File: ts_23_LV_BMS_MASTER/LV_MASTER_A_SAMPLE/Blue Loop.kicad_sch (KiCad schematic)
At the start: 16 parts, among them Q1 STD7NK40Z, Q2 STD7NK40Z, U9 ADUM3221

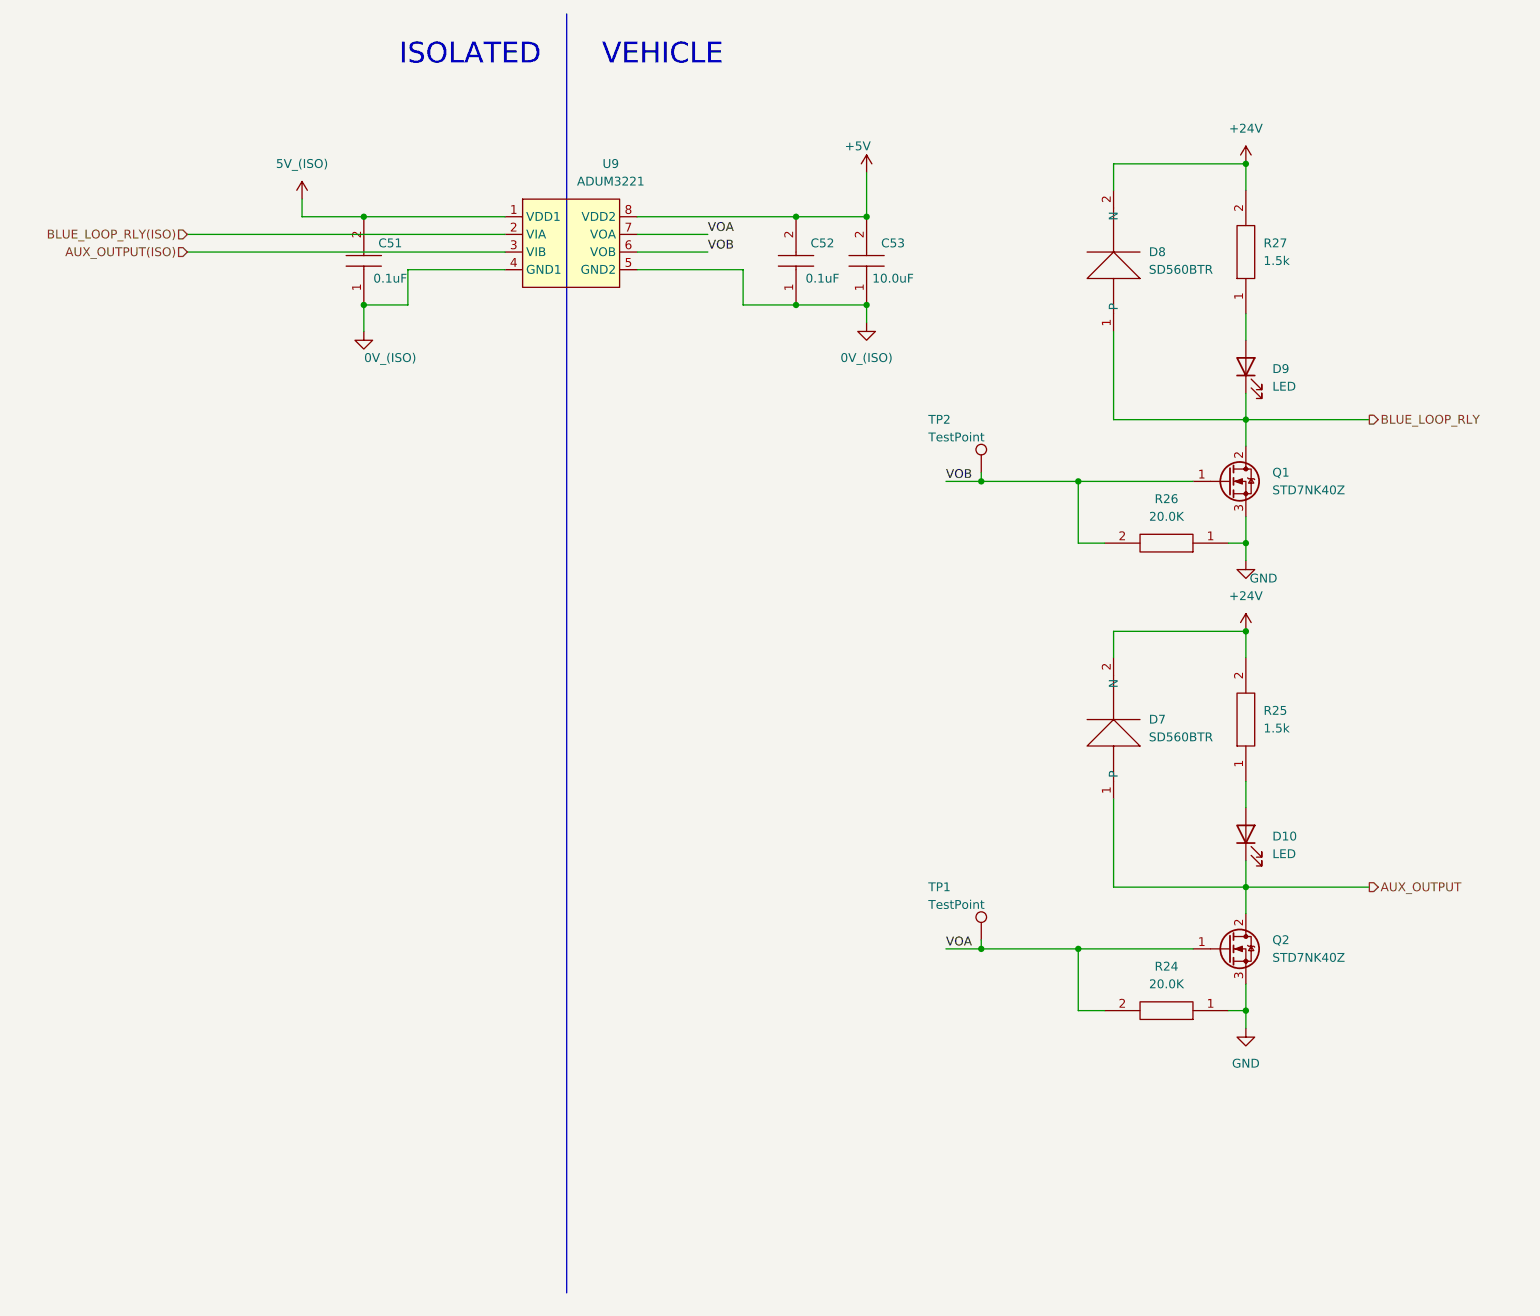
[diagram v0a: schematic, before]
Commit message: Final Changes to board
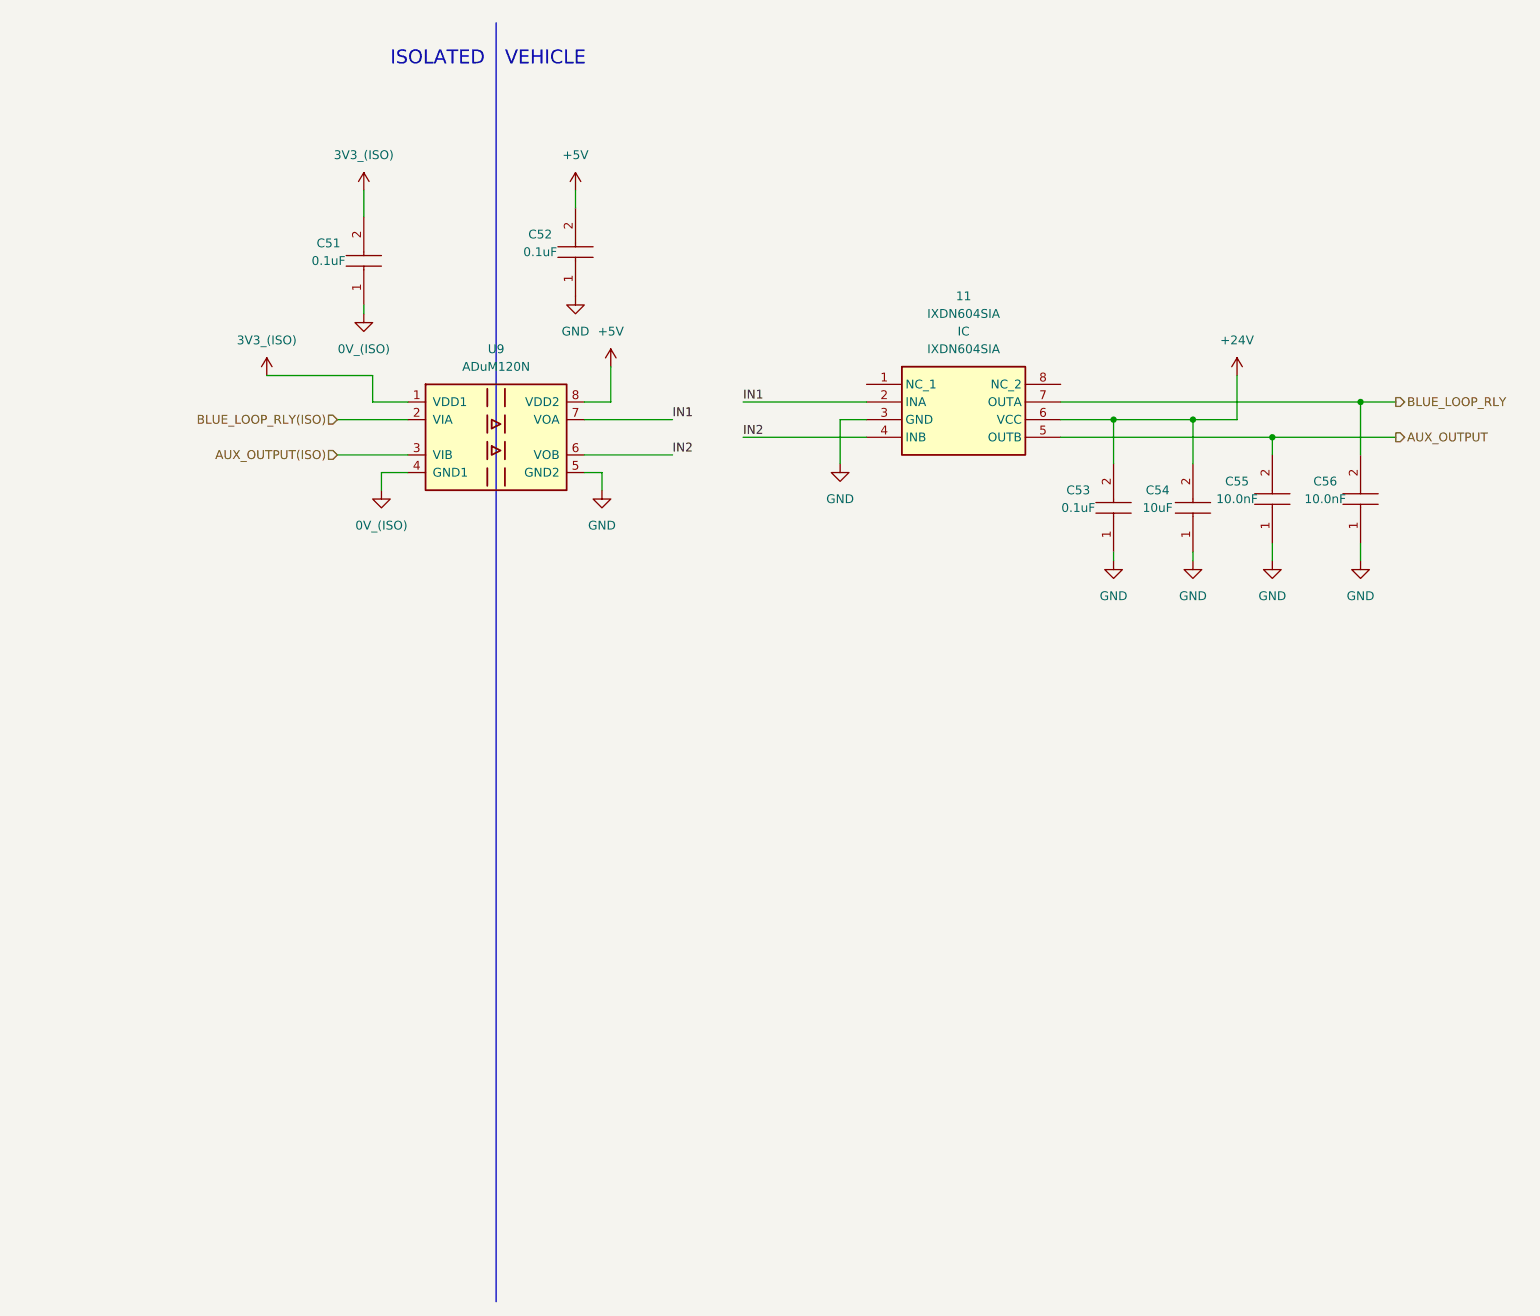
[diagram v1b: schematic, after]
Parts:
- removed D10, D9: LED, LED_SMD:LED_0805_2012Metric_Pad1.15x1.40mm_HandSolder, symbol Device:LED
- removed D7, D8: SD560BTR, Diode_SMD:D_SMB_Handsoldering, symbol Power_Protection:SD560BTR
- removed Q1, Q2: STD7NK40Z, Package_TO_SOT_SMD:TO-252-2, symbol Transistor_FET:STD7NK40Z
- removed R24, R26: 20.0K, Resistor_SMD:R_0603_1608Metric_Pad0.98x0.95mm_HandSolder, symbol ERJP06F1000V:ERJP06F1000V
- removed R25, R27: 1.5k, Resistor_SMD:R_0603_1608Metric_Pad0.98x0.95mm_HandSolder, symbol ERJP06F1000V:ERJP06F1000V
- removed TP1, TP2: TestPoint, TestPoint:TestPoint_Pad_1.0x1.0mm, symbol Connector:TestPoint
- removed U9: ADUM3221, Package_SO:SOIC-8_3.9x4.9mm_P1.27mm, symbol BMS_Library:ADUM3221
- added 11: IXDN604SIA, BMS_Library:SOIC127P600X175-8N, symbol IXDN604SIA:IXDN604SIA
- added C54: 10uF, Capacitor_SMD:C_0603_1608Metric_Pad1.08x0.95mm_HandSolder, symbol BMS_Library:CC0805JRX7R8BB104
- added C55, C56: 10.0nF, Capacitor_SMD:C_0603_1608Metric_Pad1.08x0.95mm_HandSolder, symbol BMS_Library:CC0805JRX7R8BB104
- added U9: ADuM120N, Package_SO:SOIC-8_3.9x4.9mm_P1.27mm, symbol Isolator:ADuM120N
- C53: value 10.0uF -> 0.1uF
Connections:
- net +24V: now also C53.2, 11.6 (VCC), C54.2
- net +5V: now also U9.8 (VDD2); no longer C53.2
- net 0V_(ISO): now also U9.4 (GND1)
- net AUX_OUTPUT: now also 11.5 (OUTB), C55.2
- net AUX_OUTPUT(ISO): now also U9.3 (VIB)
- net BLUE_LOOP_RLY: now also 11.7 (OUTA), C56.2
- net BLUE_LOOP_RLY(ISO): now also U9.2 (VIA)
- net GND: now also 11.3 (GND), C54.1, C55.1, C56.1, U9.5 (GND2)
- net 5V_(ISO) renamed +3.3V
- net +3.3V: now also U9.1 (VDD1)
- new net IN1: 11.2 (INA), U9.7 (VOA)
- new net IN2: 11.4 (INB), U9.6 (VOB)
